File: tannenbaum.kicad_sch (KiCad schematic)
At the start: 34 parts, among them Q1 MMBT3904-7-F, Q2 MMBT3904-7-F, Q3 MMBT3904-7-F, Q4 MMBT3904-7-F, Q5 2N7002, U1 ICM7555IPAZ

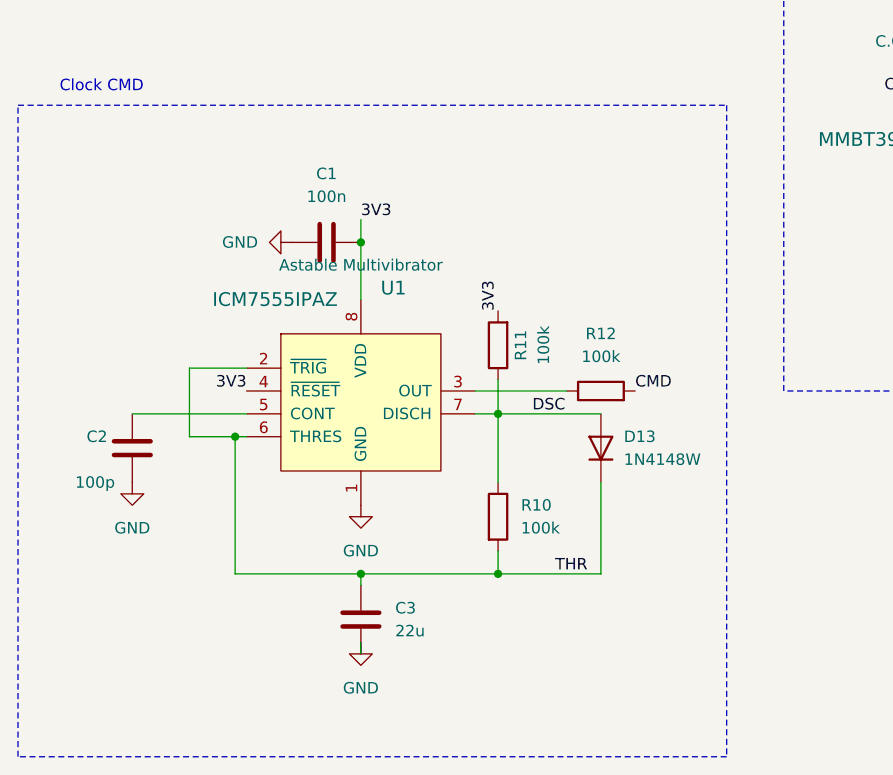
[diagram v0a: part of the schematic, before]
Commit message: pcb
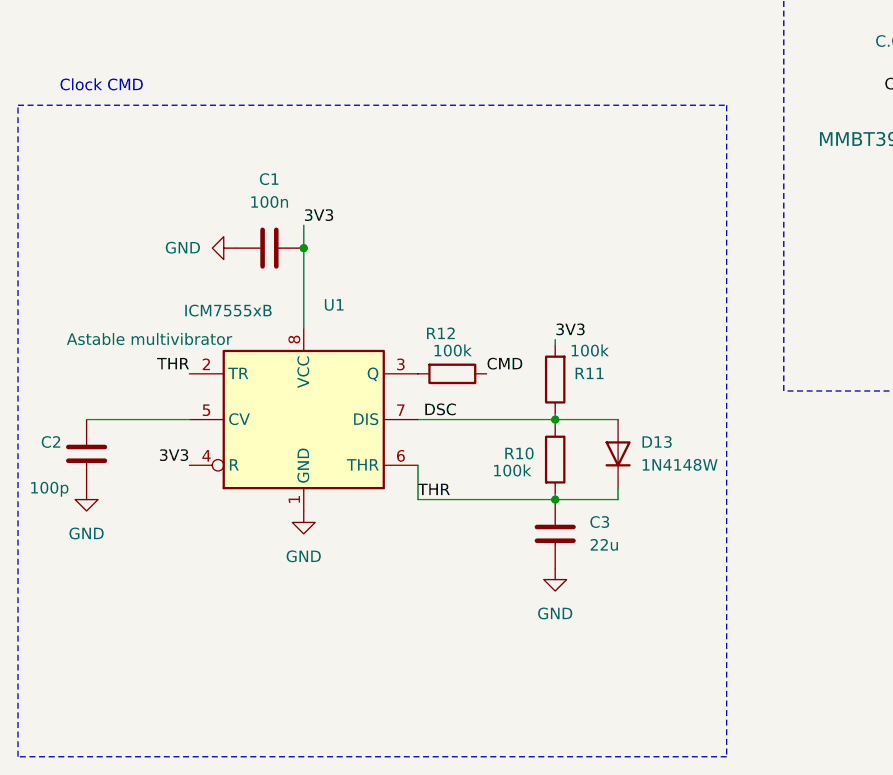
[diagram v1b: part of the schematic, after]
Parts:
- removed U1: ICM7555IPAZ, digikey-footprints:DIP-8_W7.62mm, symbol dk_Clock-Timing-Programmable-Timers-and-Oscillators:ICM7555IPAZ
- added U1: ICM7555xB, Package_SO:SOIC-8_3.9x4.9mm_P1.27mm, symbol Timer:ICM7555xB
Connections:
- net 3V3: now also U1.4 (R), U1.8 (VCC)
- net CMD: now also R12.1; no longer R12.2
- net DSC: now also U1.7 (DIS)
- net GND: now also U1.1 (GND)
- net THR: now also U1.2 (TR), U1.6 (THR)
- net at C2.1: now also U1.5 (CV)
- new net: R12.2, U1.3 (Q)
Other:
- moved on the sheet: C1, C2, C3, D13, R10, R11, R12
